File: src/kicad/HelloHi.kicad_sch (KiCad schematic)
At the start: 66 parts, among them J1 Conn_01x02, Q1 BCV29, Q2 BCV29, SW1 SW_Push, SW2 SW_Push

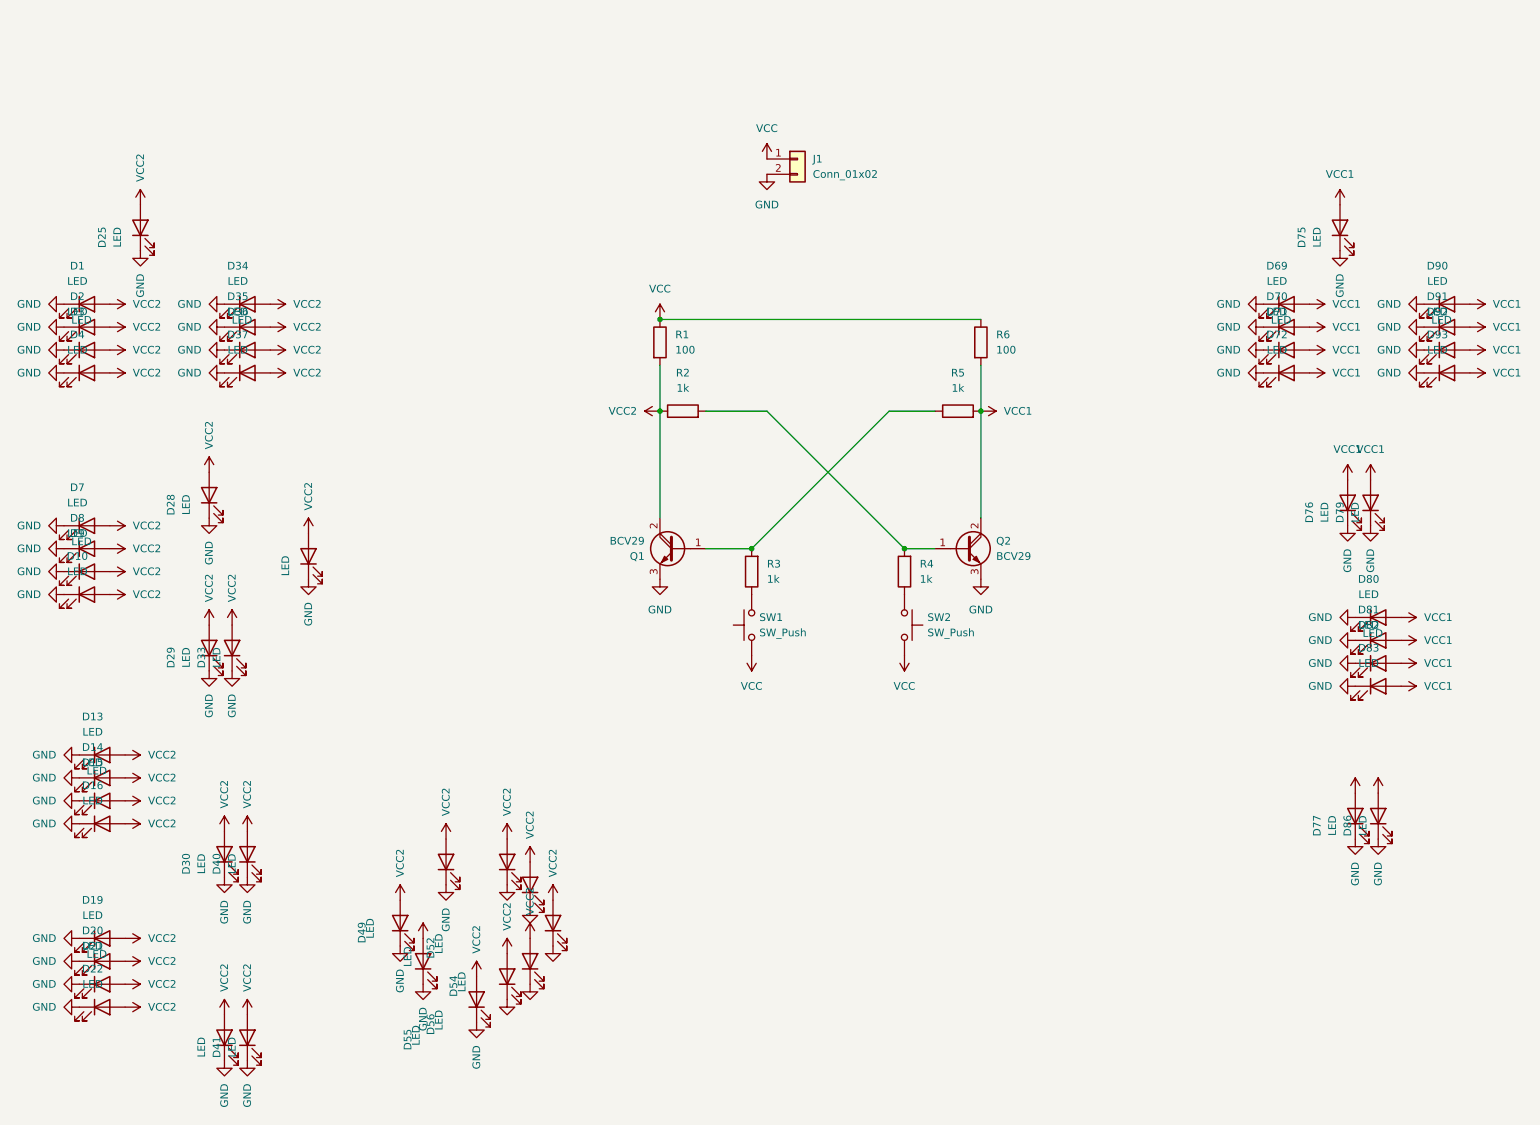
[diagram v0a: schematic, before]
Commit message: Add files via upload
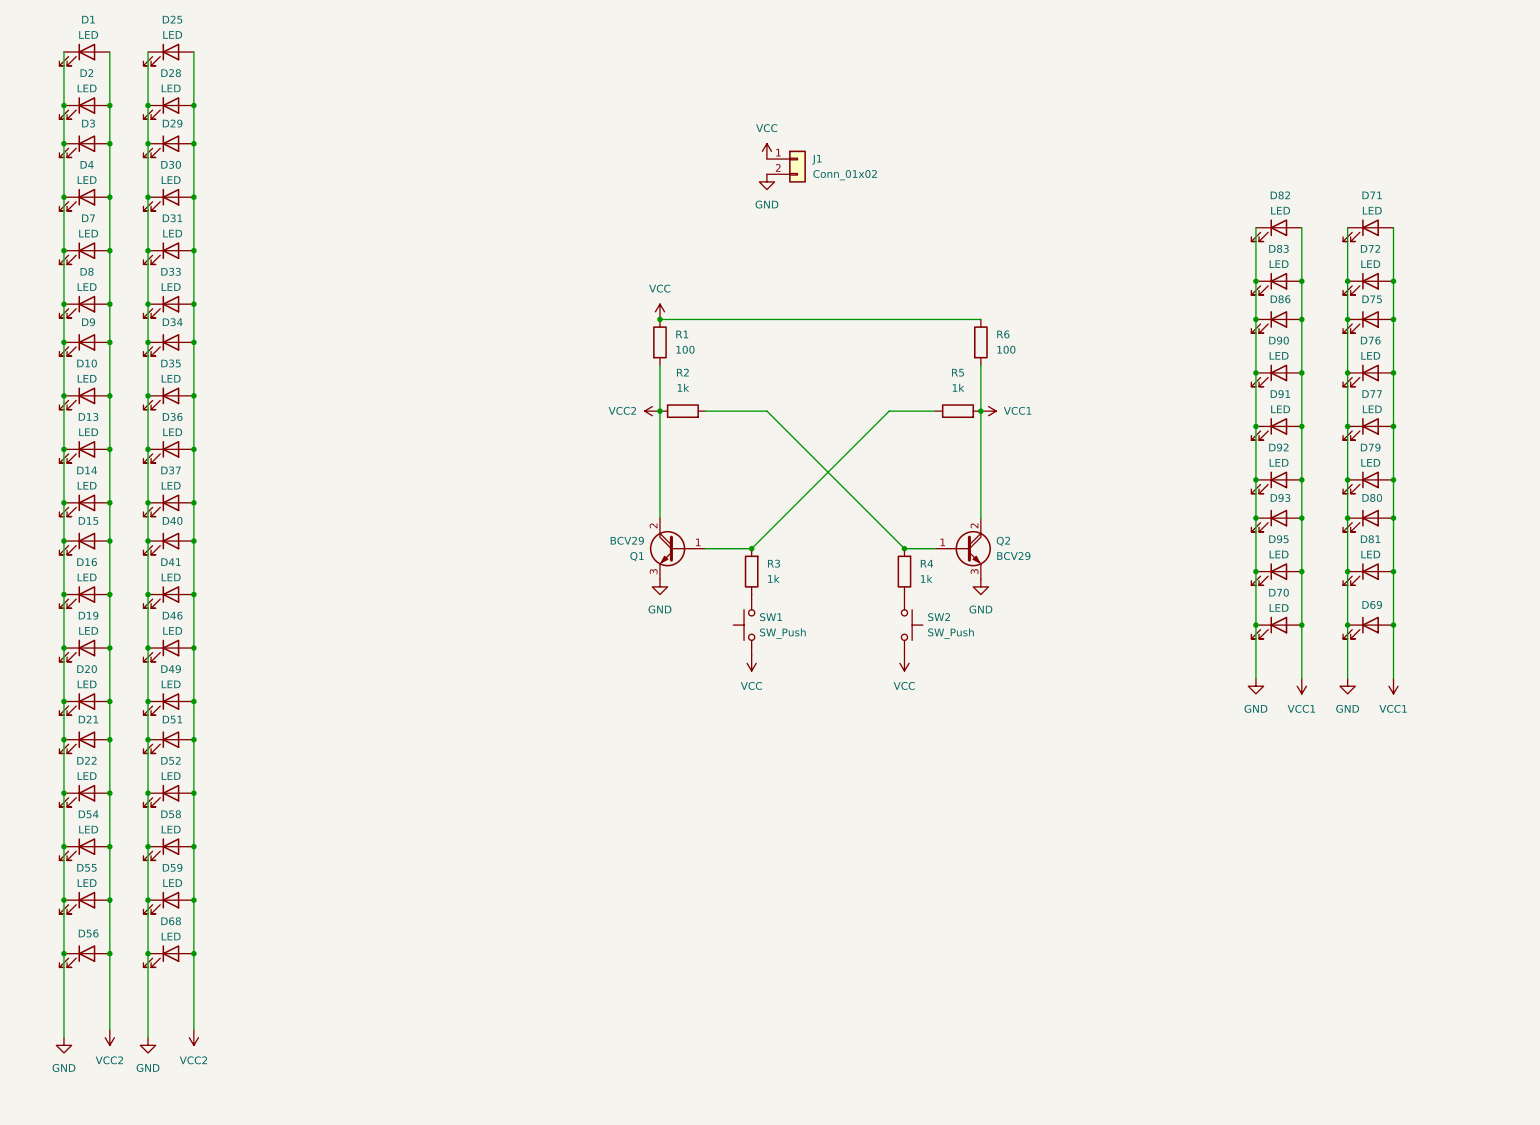
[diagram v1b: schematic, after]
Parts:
- added D95: LED, LED_THT:LED_D5.0mm, symbol Device:LED
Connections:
- net GND: now also D95.1 (K)
- net VCC1: now also D95.2 (A)
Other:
- moved on the sheet: D1, D2, D3, D4
